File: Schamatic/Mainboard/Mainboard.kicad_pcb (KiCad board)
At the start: 2 copper layers, 45 x 140 mm, 207 parts, among them J1 CONN_01X02, J10 CONN_01X04, J2 CONN_01X02, J3 CONN_01X02, J4 CONN_01X02, J5 CONN_01X02, J6 CONN_02X05, J7 CONN_02X20, J8 CONN_01X02, J9 CONN_01X02, Q1 PSMN014-40YS, Q2 PSMN014-40YS, Q3 PSMN014-40YS, Q4 PSMN014-40YS, U1 LM2678-3.3V, U10 LTC2954, U2 LM2678-5V, U4 LM5121, U6 ACS781, U7 LSM6DS33, U8 STM32F031G6U6, U9 LTC2876, Y1 Resonator_Small

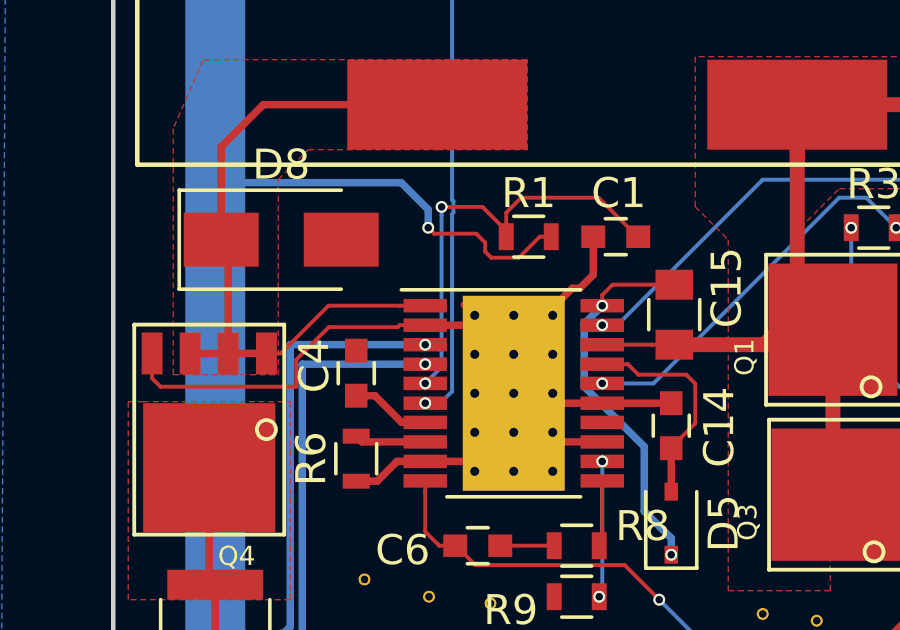
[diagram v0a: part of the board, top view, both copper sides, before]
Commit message: fixing schematic errors
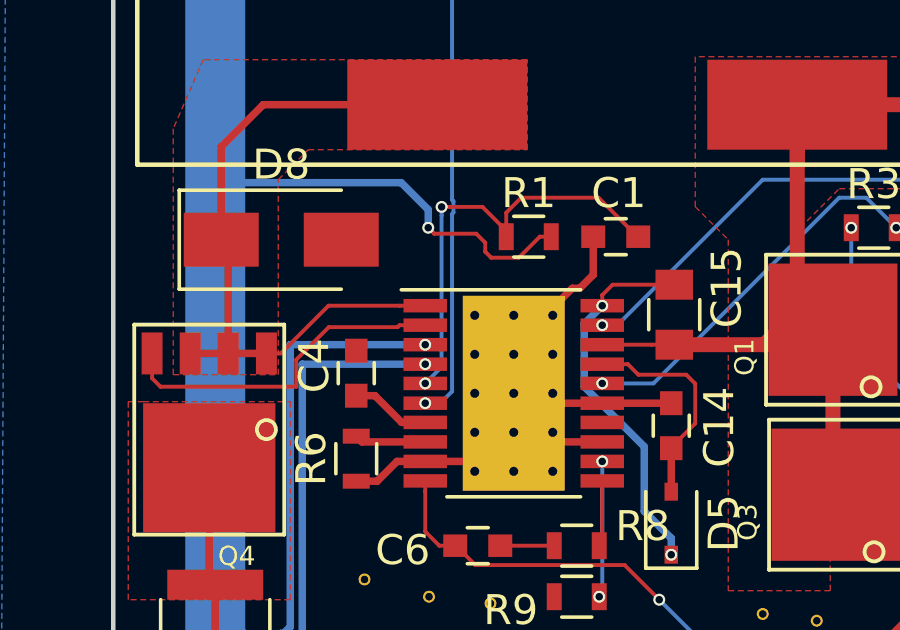
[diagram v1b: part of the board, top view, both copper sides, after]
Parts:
- C1: value 1uF -> 2.2uF
- C27: value 2.2uF -> 0.47uF
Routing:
- net Net-(Q4-Pad4): track 12.7 -> 11.4 mm
- net Earth: track 90.3 -> 89.4 mm
- added copper zone on F.Cu, net Net-(D8-Pad1)
- removed copper zone on F.Cu, net Net-(L3-Pad1)
